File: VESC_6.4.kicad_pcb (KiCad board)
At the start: 4 copper layers, 62 x 60 mm, 144 parts, among them J1 CAN, J10 SUPPLY, J11 GND, J2 HALL_ENC, J3 COMM, J4 SERVO, J5 SWD, J6 USB_OTG, J7 PH_A, J8 PH_B, J9 PH_C, Q1 IRF7749, Q2 IRF7749, Q3 IRF7749, Q4 IRF7749, Q5 IRF7749, Q6 IRF7749, SW1 SENSOR_VOLTAGE, U1 STM32F40X_LQFP64, U10 MPU9250, U2 LM3671, U3 DRV8301, U4 AD8418, U5 AD8418, U6 AD8418, U7 TJA1051TK-3, U8 NRF24L01P, U9 CONN_U.FL, Y1 Crystal_GND3, Y2 16MHz

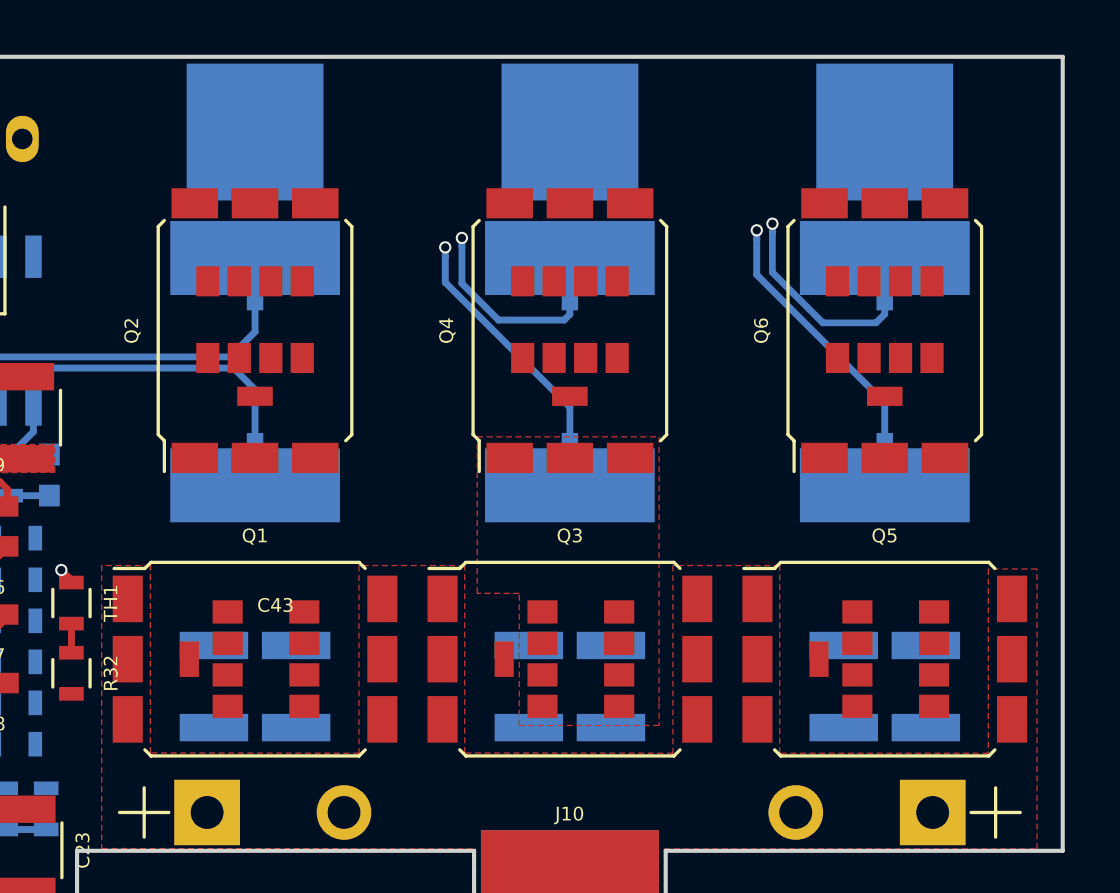
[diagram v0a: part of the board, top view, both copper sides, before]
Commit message: power electronics PCB work
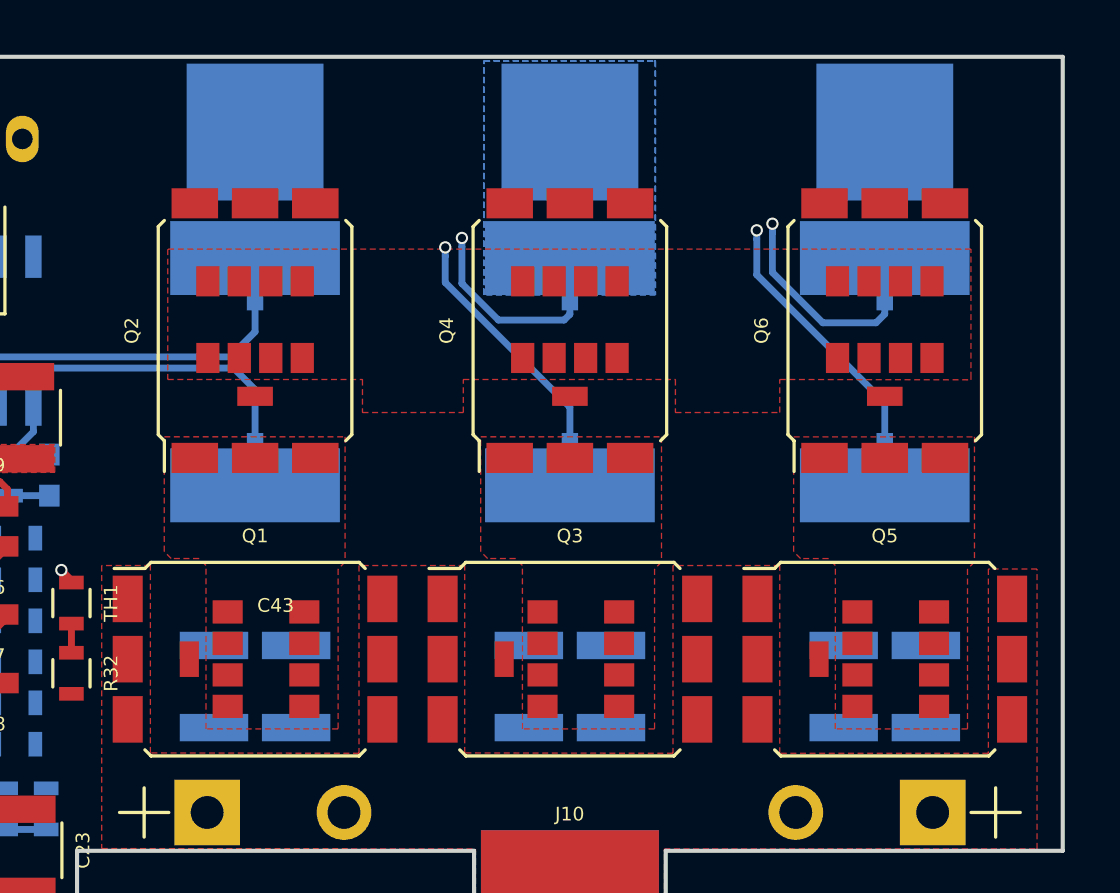
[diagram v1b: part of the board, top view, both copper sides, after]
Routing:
- added copper zone on F.Cu, net /DRV/SH_A
- added copper zone on F.Cu, net /DRV/SH_C
- added copper zone on F.Cu, net GND
- added copper zone on B.Cu, net Net-(J7-Pad1)
- added copper zone on B.Cu, net Net-(J8-Pad1)
- added copper zone on B.Cu, net Net-(J9-Pad1)
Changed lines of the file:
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@@
-(kicad_pcb (version 20170123) (host pcbnew "(2017-08-25 revision dd37d0595)-makepkg")
+(kicad_pcb (version 4) (host pcbnew 4.0.2-stable)
   (general
+    (links 454)
+    (no_connects 211)
+    (area 121.3699 61.2254 184.782401 125.8174)
     (thickness 1.6)
     (drawings 11)
@@
       (hpglpenspeed 20)
       (hpglpendiameter 15)
+      (hpglpenoverlay 2)
       (psnegative false)
       (psa4output false)
@@
     (at 138.7983 84.8741 270)
     (attr smd)
-    (fp_text reference U3 (at -8.4 0) (layer F.SilkS)
+    (fp_text reference U3 (at -8.4 0 360) (layer F.SilkS)
       (effects (font (size 0.5 0.5) (thickness 0.125)))
     )
@@
     (tags "capacitor 0603")
     (attr smd)
-    (fp_text reference C55 (at 1.75115 0.00898 45) (layer F.SilkS)
+    (fp_text reference C55 (at 1.75115 0.00898 405) (layer F.SilkS)
       (effects (font (size 0.5 0.5) (thickness 0.125)))
     )
@@
     (tags "resistor 0603")
     (attr smd)
-    (fp_text reference R29 (at -1.651 -0.0254 90) (layer B.SilkS)
+    (fp_text reference R29 (at -1.651 -0.0254 450) (layer B.SilkS)
       (effects (font (size 0.5 0.5) (thickness 0.125)) (justify mirror))
     )
-    (fp_text value 4.7 (at 1.5875 -0.0254 90) (layer B.Fab)
+    (fp_text value 4.7 (at 1.5875 -0.0254 450) (layer B.Fab)
       (effects (font (size 0.5 0.5) (thickness 0.125)) (justify mirror))
     )
@@
     (tags "resistor 0603")
     (attr smd)
-    (fp_text reference R30 (at -1.6764 -0.0127 90) (layer B.SilkS)
+    (fp_text reference R30 (at -1.6764 -0.0127 450) (layer B.SilkS)
       (effects (font (size 0.5 0.5) (thickness 0.125)) (justify mirror))
     )
-    (fp_text value 4.7 (at 1.6002 0 90) (layer B.Fab)
+    (fp_text value 4.7 (at 1.6002 0 450) (layer B.Fab)
       (effects (font (size 0.5 0.5) (thickness 0.125)) (justify mirror))
     )
@@
     (tags "resistor 0603")
     (attr smd)
-    (fp_text reference R33 (at -1.6637 0 90) (layer B.SilkS)
+    (fp_text reference R33 (at -1.6637 0 450) (layer B.SilkS)
       (effects (font (size 0.5 0.5) (thickness 0.125)) (justify mirror))
     )
-    (fp_text value 4.7 (at 1.6256 -0.0127 90) (layer B.Fab)
+    (fp_text value 4.7 (at 1.6256 -0.0127 450) (layer B.Fab)
       (effects (font (size 0.5 0.5) (thickness 0.125)) (justify mirror))
     )
@@
     (tags "resistor 0603")
     (attr smd)
-    (fp_text reference R34 (at -1.6764 0 90) (layer B.SilkS)
+    (fp_text reference R34 (at -1.6764 0 450) (layer B.SilkS)
       (effects (font (size 0.5 0.5) (thickness 0.125)) (justify mirror))
     )
-    (fp_text value 4.7 (at 1.6256 -0.0127 90) (layer B.Fab)
+    (fp_text value 4.7 (at 1.6256 -0.0127 450) (layer B.Fab)
       (effects (font (size 0.5 0.5) (thickness 0.125)) (justify mirror))
     )
@@
     (tags "resistor 0603")
     (attr smd)
-    (fp_text reference R36 (at -1.651 0 90) (layer B.SilkS)
+    (fp_text reference R36 (at -1.651 0 450) (layer B.SilkS)
       (effects (font (size 0.5 0.5) (thickness 0.125)) (justify mirror))
     )
-    (fp_text value 4.7 (at 1.6002 -0.0381 90) (layer B.Fab)
+    (fp_text value 4.7 (at 1.6002 -0.0381 450) (layer B.Fab)
       (effects (font (size 0.5 0.5) (thickness 0.125)) (justify mirror))
     )
@@
     (tags "resistor 0603")
     (attr smd)
-    (fp_text reference R37 (at 1.6637 -0.0127 90) (layer B.SilkS)
+    (fp_text reference R37 (at 1.6637 -0.0127 450) (layer B.SilkS)
       (effects (font (size 0.5 0.5) (thickness 0.125)) (justify mirror))
     )
-    (fp_text value 4.7 (at -1.6383 -0.0127 90) (layer B.Fab)
+    (fp_text value 4.7 (at -1.6383 -0.0127 450) (layer B.Fab)
       (effects (font (size 0.5 0.5) (thickness 0.125)) (justify mirror))
     )
@@
       (effects (font (size 0.5 0.5) (thickness 0.125)))
     )
-    (fp_text value NRF24L01P (at 7.830783 -8.046309 45) (layer F.Fab)
+    (fp_text value NRF24L01P (at 7.830783 -8.046309 405) (layer F.Fab)
       (effects (font (size 0.5 0.5) (thickness 0.125)))
     )
@@
     (fp_line (start 0.9 1.61) (end -1.55 1.61) (layer B.SilkS) (width 0.12))
     (fp_line (start -0.9 -1.61) (end 0.9 -1.61) (layer B.SilkS) (width 0.12))
-    (fp_text user %R (at 0 0 90) (layer B.Fab)
+    (fp_text user %R (at 0 0 450) (layer B.Fab)
       (effects (font (size 0.5 0.5) (thickness 0.125)) (justify mirror))
     )
@@
     )
   )
+  (zone (net 25) (net_name /DRV/SH_C) (layer F.Cu) (hatch edge 0.508)
+    (connect_pads yes (clearance 0.1))
+    (min_thickness 0.254)
+    (fill yes (arc_segments 16) (thermal_gap 0.508) (thermal_bridge_width 0.508))
+    (polygon
+      (pts
+        (xy 181.483 78.486) (xy 181.483 83.058) (xy 181.229 83.312) (xy 181.229 89.154) (xy 176.403 89.154)
+        (xy 176.403 88.4301) (xy 176.403 83.185) (xy 176.149 82.931) (xy 175.133 82.931) (xy 174.879 82.677)
+        (xy 174.879 78.486)
+      )
+    )
+  )
+  (zone (net 21) (net_name /DRV/SH_A) (layer F.Cu) (hatch edge 0.508)
+    (connect_pads yes (clearance 0.1))
+    (min_thickness 0.254)
+    (fill yes (arc_segments 16) (thermal_gap 0.508) (thermal_bridge_width 0.508))
+    (polygon
+      (pts
+        (xy 158.496 78.484748) (xy 158.496 83.056748) (xy 158.242 83.310748) (xy 158.242 89.152748) (xy 153.416 89.152748)
+        (xy 153.416 88.428848) (xy 153.416 83.183748) (xy 153.162 82.929748) (xy 152.146 82.929748) (xy 151.892 82.675748)
+        (xy 151.892 78.484748)
+      )
+    )
+  )
   (zone (net 22) (net_name /DRV/SH_B) (layer F.Cu) (hatch edge 0.508)
     (connect_pads yes (clearance 0.1))
-    (min_thickness 1)
+    (min_thickness 0.254)
+    (fill yes (arc_segments 16) (thermal_gap 0.508) (thermal_bridge_width 0.508))
+    (polygon
+      (pts
+        (xy 170.053 78.484748) (xy 170.053 83.056748) (xy 169.799 83.310748) (xy 169.799 89.152748) (xy 164.973 89.152748)
+        (xy 164.973 88.428848) (xy 164.973 83.183748) (xy 164.719 82.929748) (xy 163.703 82.929748) (xy 163.449 82.675748)
+        (xy 163.449 78.484748)
+      )
+    )
+  )
+  (zone (net 2) (net_name GND) (layer F.Cu) (hatch edge 0.508)
+    (connect_pads yes (clearance 0.1))
+    (min_thickness 0.254)
+    (fill yes (arc_segments 16) (thermal_gap 0.508) (thermal_bridge_width 0.508))
+    (polygon
+      (pts
+        (xy 181.356 76.327) (xy 181.356 71.628) (xy 152.019 71.628) (xy 152.019 76.3905) (xy 159.131 76.3905)
+        (xy 159.131 77.597) (xy 162.814 77.597) (xy 162.814 76.5175) (xy 162.814 76.3905) (xy 170.561 76.3905)
+        (xy 170.561 77.597) (xy 174.371 77.597) (xy 174.371 76.3905) (xy 181.356 76.4032)
+      )
+    )
+  )
+  (zone (net 137) (net_name "Net-(J8-Pad1)") (layer B.Cu) (hatch edge 0.508)
+    (connect_pads yes (clearance 0.1))
+    (min_thickness 0.254)
+    (fill yes (arc_segments 16) (thermal_gap 0.508) (thermal_bridge_width 0.508))
+    (polygon
+      (pts
+        (xy 163.576 73.3044) (xy 163.576 70.485) (xy 163.576 64.77) (xy 169.799 64.77) (xy 169.8371 64.77)
+        (xy 169.8371 73.3044)
+      )
+    )
+  )
+  (zone (net 136) (net_name "Net-(J7-Pad1)") (layer B.Cu) (hatch edge 0.508)
+    (connect_pads yes (clearance 0.1))
+    (min_thickness 0.254)
+    (fill yes (arc_segments 16) (thermal_gap 0.508) (thermal_bridge_width 0.508))
+    (polygon
+      (pts
+        (xy 163.5633 73.279003) (xy 163.5633 70.459603) (xy 163.5633 64.744603) (xy 169.7863 64.744603) (xy 169.8244 64.744603)
+        (xy 169.8244 73.279003)
+      )
+    )
+  )
+  (zone (net 138) (net_name "Net-(J9-Pad1)") (layer B.Cu) (hatch edge 0.508)
+    (connect_pads yes (clearance 0.1))
+    (min_thickness 0.254)
     (fill yes (arc_segments 16) (thermal_gap 0.508) (thermal_bridge_width 0.508))
     (polygon
       (pts
-        (xy 169.9641 78.4987) (xy 169.9641 88.2142) (xy 169.9641 89.027) (xy 164.8587 89.027) (xy 164.8587 84.201)
-        (xy 163.322 84.201) (xy 163.322 78.486) (xy 169.9641 78.486)
+        (xy 163.5633 73.286983) (xy 163.5633 70.467583) (xy 163.5633 64.752583) (xy 169.7863 64.752583) (xy 169.8244 64.752583)
+        (xy 169.8244 73.286983)
       )
     )
